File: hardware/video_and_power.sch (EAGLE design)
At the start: 37 parts, among them IC1 74HCT574N, IC2 74HCT574N, IC3 74HCT574N, IC4 74HCT04N, IC5 7432N, IC7 7805T, J2 POWER_JACKSLT, X1 736880-49

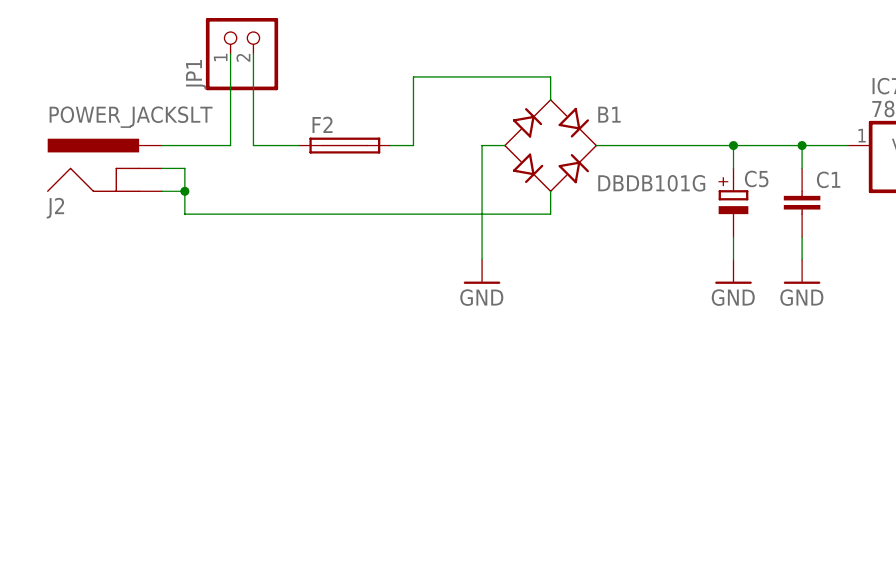
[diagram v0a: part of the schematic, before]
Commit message: PCB update
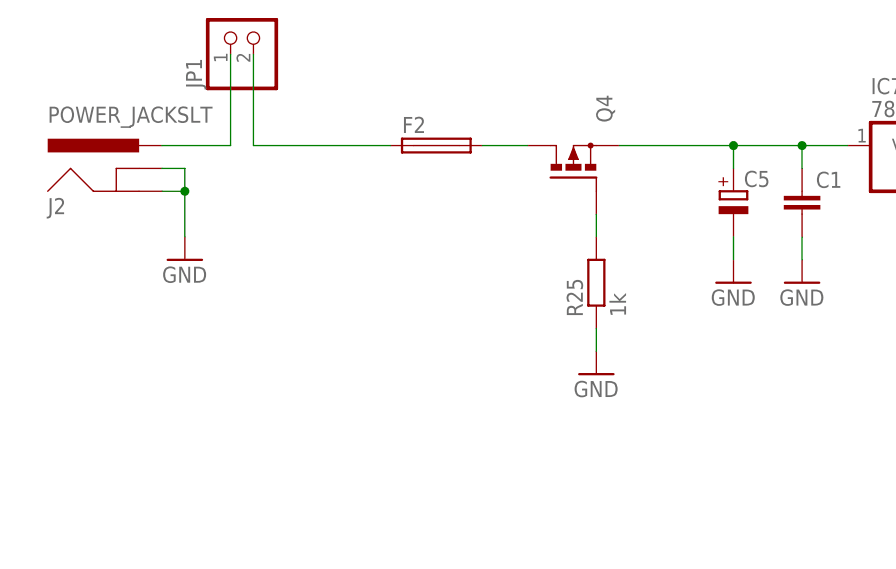
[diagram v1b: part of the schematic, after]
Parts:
- removed B1: DBDB101G, rectifier:DBDB101G
- added Q4: (no value), transistor-power:P-MOSFET-SO8
- added R25: 1k, rcl:R-EU_R0603
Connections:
- removed net N$12: B1.AC2, J2.GND, J2.GNDBREAK
- removed net N$14: B1.+, C1.1, C5.+, IC7.VI
- new net 9V: C1.1, C5.+, IC7.VI, Q4.S
- new net N$52: F2.2, Q4.D
- net GND: now also J2.GND, J2.GNDBREAK, R25.1; no longer B1.-
- net N$3: now also Q4.G, R25.2; no longer B1.AC1, F2.2
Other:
- moved on the sheet: F2
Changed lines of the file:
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@@
 <layer number="154" name="FabDoc2" color="7" fill="1" visible="yes" active="yes"/>
 <layer number="155" name="FabDoc3" color="7" fill="1" visible="yes" active="yes"/>
+<layer number="156" name="gesam-Maß" color="1" fill="7" visible="no" active="no"/>
+<layer number="157" name="FaceMchng" color="3" fill="1" visible="no" active="no"/>
+<layer number="158" name="FaceMMeas" color="3" fill="1" visible="no" active="no"/>
+<layer number="159" name="Geh-Bear2" color="1" fill="7" visible="no" active="no"/>
+<layer number="160" name="Topologie" color="9" fill="1" visible="no" active="no"/>
+<layer number="161" name="tomplace2" color="7" fill="1" visible="no" active="no"/>
 <layer number="191" name="mNets" color="7" fill="1" visible="yes" active="yes"/>
 <layer number="192" name="mBusses" color="7" fill="1" visible="yes" active="yes"/>
@@
 <layer number="250" name="Descript" color="3" fill="1" visible="no" active="no"/>
 <layer number="251" name="SMDround" color="12" fill="11" visible="no" active="no"/>
+<layer number="252" name="BR-BS" color="7" fill="1" visible="no" active="no"/>
+<layer number="253" name="BR-LS" color="7" fill="1" visible="no" active="no"/>
 <layer number="254" name="cooling" color="7" fill="1" visible="yes" active="yes"/>
 <layer number="255" name="HELP" color="7" fill="1" visible="yes" active="yes"/>
@@
 <part name="IC4" library="74xx-eu" deviceset="74*04" device="N" technology="HCT"/>
 <part name="J2" library="SparkFun-Connectors" deviceset="POWER_JACK" device="SLT"/>
-<part name="GND7" library="supply1" deviceset="GND" device=""/>
 <part name="IC7" library="linear" deviceset="78*" device="T" technology="05"/>
 <part name="GND8" library="supply1" deviceset="GND" device=""/>
@@
 <part name="C4" library="rcl" deviceset="C-EU" device="C0603"/>
 <part name="GND12" library="supply1" deviceset="GND" device=""/>
-<part name="B1" library="rectifier" deviceset="DB?*G" device="DB10" technology="1"/>
 <part name="GND14" library="supply1" deviceset="GND" device=""/>
 <part name="GND15" library="supply1" deviceset="GND" device=""/>
@@
 <part name="IC5" library="74xx-us" deviceset="74*32" device="N"/>
 <part name="GND18" library="supply1" deviceset="GND" device=""/>
+<part name="Q4" library="transistor-power" deviceset="P-MOSFET-SO8" device=""/>
+<part name="R25" library="rcl" deviceset="R-EU_" device="R0603" value="1k"/>
+<part name="GND7" library="supply1" deviceset="GND" device=""/>
+<part name="GND19" library="supply1" deviceset="GND" device=""/>
 </parts>
 <sheets>
@@
 <instance part="IC4" gate="P" x="266.7" y="137.16"/>
 <instance part="J2" gate="G$1" x="83.82" y="190.5"/>
-<instance part="GND7" gate="1" x="121.92" y="182.88"/>
 <instance part="IC7" gate="A1" x="172.72" y="198.12"/>
 <instance part="GND8" gate="1" x="172.72" y="182.88"/>
-<instance part="F2" gate="1" x="106.68" y="198.12"/>
+<instance part="F2" gate="1" x="116.84" y="198.12"/>
 <instance part="X1" gate="G$1" x="50.8" y="-25.4" rot="MR0"/>
 <instance part="GND9" gate="1" x="45.72" y="-43.18"/>
@@
 <instance part="C4" gate="G$1" x="43.18" y="0" rot="R90"/>
 <instance part="GND12" gate="1" x="50.8" y="-5.08"/>
-<instance part="B1" gate="G$1" x="129.54" y="198.12"/>
 <instance part="GND14" gate="1" x="157.48" y="182.88"/>
 <instance part="GND15" gate="1" x="185.42" y="182.88"/>
@@
 <instance part="IC5" gate="D" x="340.36" y="-22.86"/>
 <instance part="GND18" gate="1" x="401.32" y="-30.48"/>
+<instance part="Q4" gate="G$1" x="132.08" y="195.58" rot="MR90"/>
+<instance part="R25" gate="G$1" x="134.62" y="182.88" rot="R90"/>
+<instance part="GND7" gate="1" x="134.62" y="172.72"/>
+<instance part="GND19" gate="1" x="88.9" y="185.42"/>
 </instances>
 <busses>
@@
 </segment>
 <segment>
-<pinref part="B1" gate="G$1" pin="-"/>
-<wire x1="124.46" y1="198.12" x2="121.92" y2="198.12" width="0.1524" layer="91"/>
-<wire x1="121.92" y1="198.12" x2="121.92" y2="185.42" width="0.1524" layer="91"/>
-<pinref part="GND7" gate="1" pin="GND"/>
-</segment>
-<segment>
 <pinref part="C1" gate="G$1" pin="2"/>
 <pinref part="GND14" gate="1" pin="GND"/>
@@
 <junction x="401.32" y="0"/>
 </segment>
+<segment>
+<pinref part="GND7" gate="1" pin="GND"/>
+<pinref part="R25" gate="G$1" pin="1"/>
+<wire x1="134.62" y1="175.26" x2="134.62" y2="177.8" width="0.1524" layer="91"/>
+</segment>
+<segment>
+<pinref part="J2" gate="G$1" pin="GNDBREAK"/>
+<wire x1="86.36" y1="195.58" x2="88.9" y2="195.58" width="0.1524" layer="91"/>
+<wire x1="88.9" y1="195.58" x2="88.9" y2="193.04" width="0.1524" layer="91"/>
+<pinref part="J2" gate="G$1" pin="GND"/>
+<wire x1="88.9" y1="193.04" x2="86.36" y2="193.04" width="0.1524" layer="91"/>
+<wire x1="88.9" y1="193.04" x2="88.9" y2="187.96" width="0.1524" layer="91"/>
+<junction x="88.9" y="193.04"/>
+<pinref part="GND19" gate="1" pin="GND"/>
+</segment>
 </net>
 <net name="D0" class="0">
@@
 </segment>
 </net>
-<net name="N$12" class="0">
-<segment>
-<pinref part="J2" gate="G$1" pin="GNDBREAK"/>
-<wire x1="86.36" y1="195.58" x2="88.9" y2="195.58" width="0.1524" layer="91"/>
-<wire x1="88.9" y1="195.58" x2="88.9" y2="193.04" width="0.1524" layer="91"/>
-<pinref part="J2" gate="G$1" pin="GND"/>
-<wire x1="88.9" y1="193.04" x2="86.36" y2="193.04" width="0.1524" layer="91"/>
-<wire x1="88.9" y1="193.04" x2="88.9" y2="190.5" width="0.1524" layer="91"/>
-<junction x="88.9" y="193.04"/>
-<pinref part="B1" gate="G$1" pin="AC2"/>
-<wire x1="88.9" y1="190.5" x2="129.54" y2="190.5" width="0.1524" layer="91"/>
-<wire x1="129.54" y1="190.5" x2="129.54" y2="193.04" width="0.1524" layer="91"/>
-</segment>
-</net>
-<net name="N$3" class="0">
-<segment>
-<wire x1="114.3" y1="198.12" x2="114.3" y2="205.74" width="0.1524" layer="91"/>
-<pinref part="B1" gate="G$1" pin="AC1"/>
-<wire x1="114.3" y1="205.74" x2="129.54" y2="205.74" width="0.1524" layer="91"/>
-<wire x1="129.54" y1="205.74" x2="129.54" y2="203.2" width="0.1524" layer="91"/>
-<pinref part="F2" gate="1" pin="2"/>
-<wire x1="111.76" y1="198.12" x2="114.3" y2="198.12" width="0.1524" layer="91"/>
-</segment>
-</net>
-<net name="N$14" class="0">
-<segment>
-<pinref part="B1" gate="G$1" pin="+"/>
+<net name="N$8" class="0">
+<segment>
+<pinref part="J2" gate="G$1" pin="PWR"/>
+<pinref part="JP1" gate="G$1" pin="1"/>
+<wire x1="86.36" y1="198.12" x2="93.98" y2="198.12" width="0.1524" layer="91"/>
+<wire x1="93.98" y1="198.12" x2="93.98" y2="208.28" width="0.1524" layer="91"/>
+</segment>
+</net>
+<net name="N$13" class="0">
+<segment>
+<pinref part="JP1" gate="G$1" pin="2"/>
+<wire x1="96.52" y1="208.28" x2="96.52" y2="198.12" width="0.1524" layer="91"/>
+<pinref part="F2" gate="1" pin="1"/>
+<wire x1="96.52" y1="198.12" x2="111.76" y2="198.12" width="0.1524" layer="91"/>
+</segment>
+</net>
+<net name="9V" class="0">
+<segment>
+<wire x1="137.16" y1="198.12" x2="149.86" y2="198.12" width="0.1524" layer="91"/>
+<pinref part="Q4" gate="G$1" pin="S"/>
 <pinref part="IC7" gate="A1" pin="VI"/>
-<wire x1="134.62" y1="198.12" x2="149.86" y2="198.12" width="0.1524" layer="91"/>
 <pinref part="C1" gate="G$1" pin="1"/>
 <wire x1="149.86" y1="198.12" x2="157.48" y2="198.12" width="0.1524" layer="91"/>
@@
 </segment>
 </net>
-<net name="N$8" class="0">
-<segment>
-<pinref part="J2" gate="G$1" pin="PWR"/>
-<pinref part="JP1" gate="G$1" pin="1"/>
-<wire x1="86.36" y1="198.12" x2="93.98" y2="198.12" width="0.1524" layer="91"/>
-<wire x1="93.98" y1="198.12" x2="93.98" y2="208.28" width="0.1524" layer="91"/>
-</segment>
-</net>
-<net name="N$13" class="0">
-<segment>
-<pinref part="JP1" gate="G$1" pin="2"/>
-<wire x1="96.52" y1="208.28" x2="96.52" y2="198.12" width="0.1524" layer="91"/>
-<pinref part="F2" gate="1" pin="1"/>
-<wire x1="96.52" y1="198.12" x2="101.6" y2="198.12" width="0.1524" layer="91"/>
-</segment>
-</net>
+<net name="N$52" class="0">
+<segment>
+<pinref part="Q4" gate="G$1" pin="D"/>
+<wire x1="127" y1="198.12" x2="121.92" y2="198.12" width="0.1524" layer="91"/>
+<pinref part="F2" gate="1" pin="2"/>
+</segment>
+</net>
+<net name="N$3" class="0">
+<segment>
+<pinref part="Q4" gate="G$1" pin="G"/>
+<pinref part="R25" gate="G$1" pin="2"/>
+<wire x1="134.62" y1="187.96" x2="134.62" y2="190.5" width="0.1524" layer="91"/>
+</segment>
+</net>
